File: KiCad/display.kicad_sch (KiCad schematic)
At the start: 30 parts, among them IC2 R1200N001A-TR-FE, J3 Conn_01x34_NHD_18, Q3 DMG2302U, Q4 DMG2302U, U6 MCP1700x-250xxTT

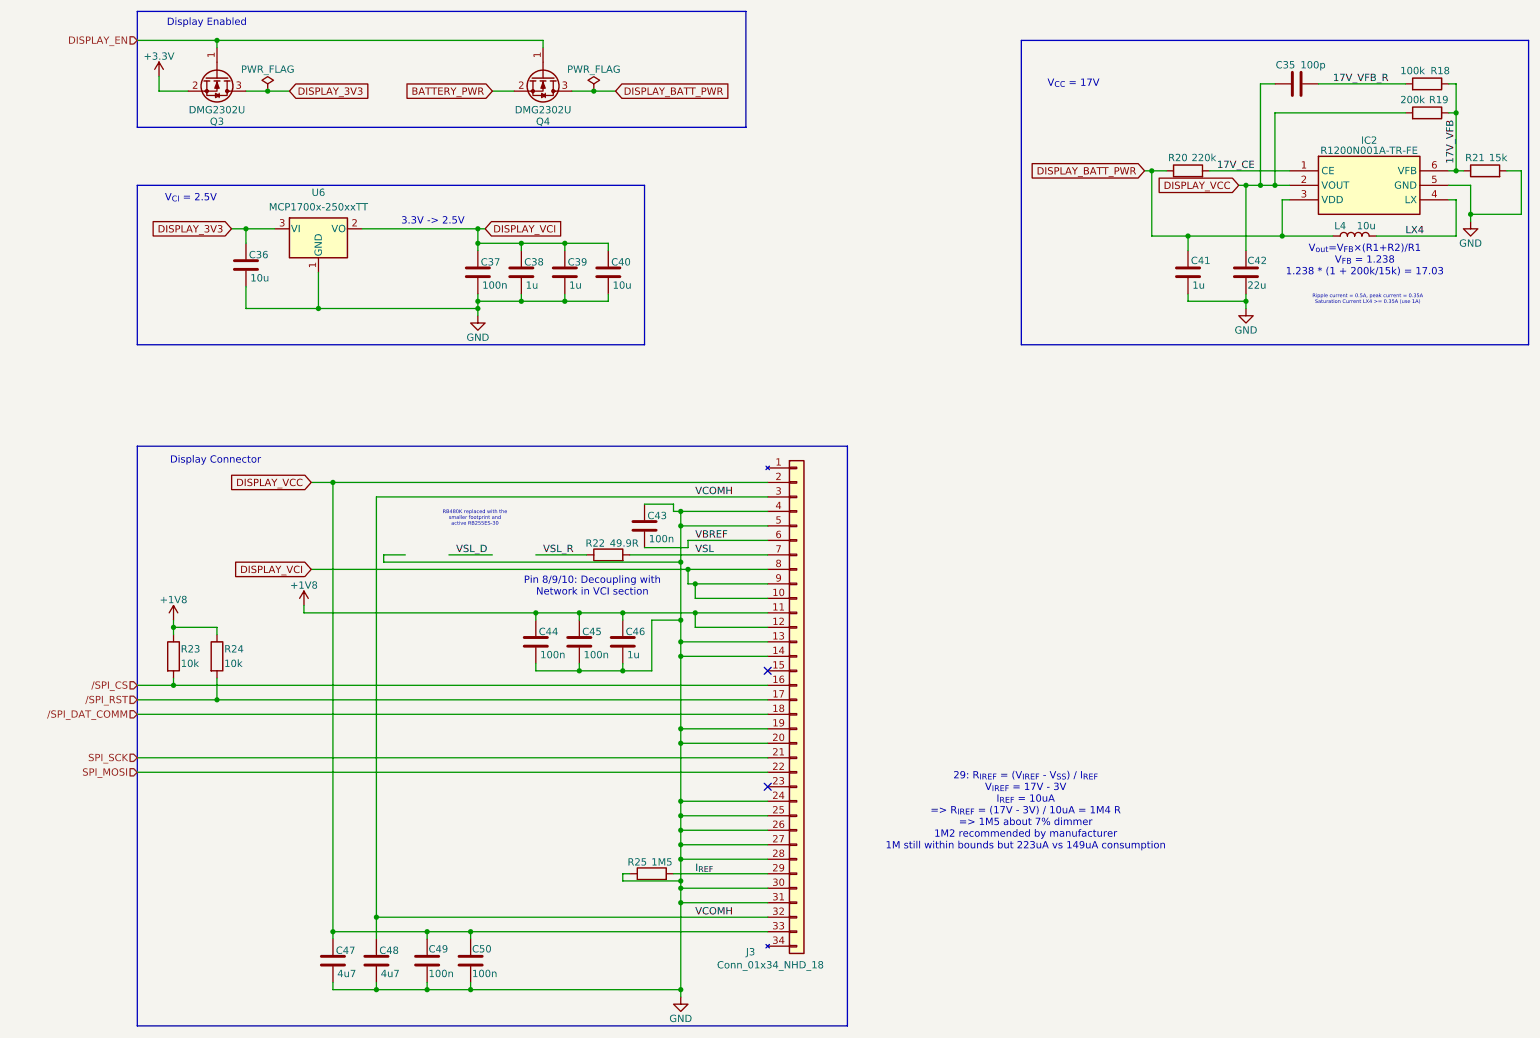
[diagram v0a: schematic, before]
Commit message: Implement Comments, Working on PCB Layout
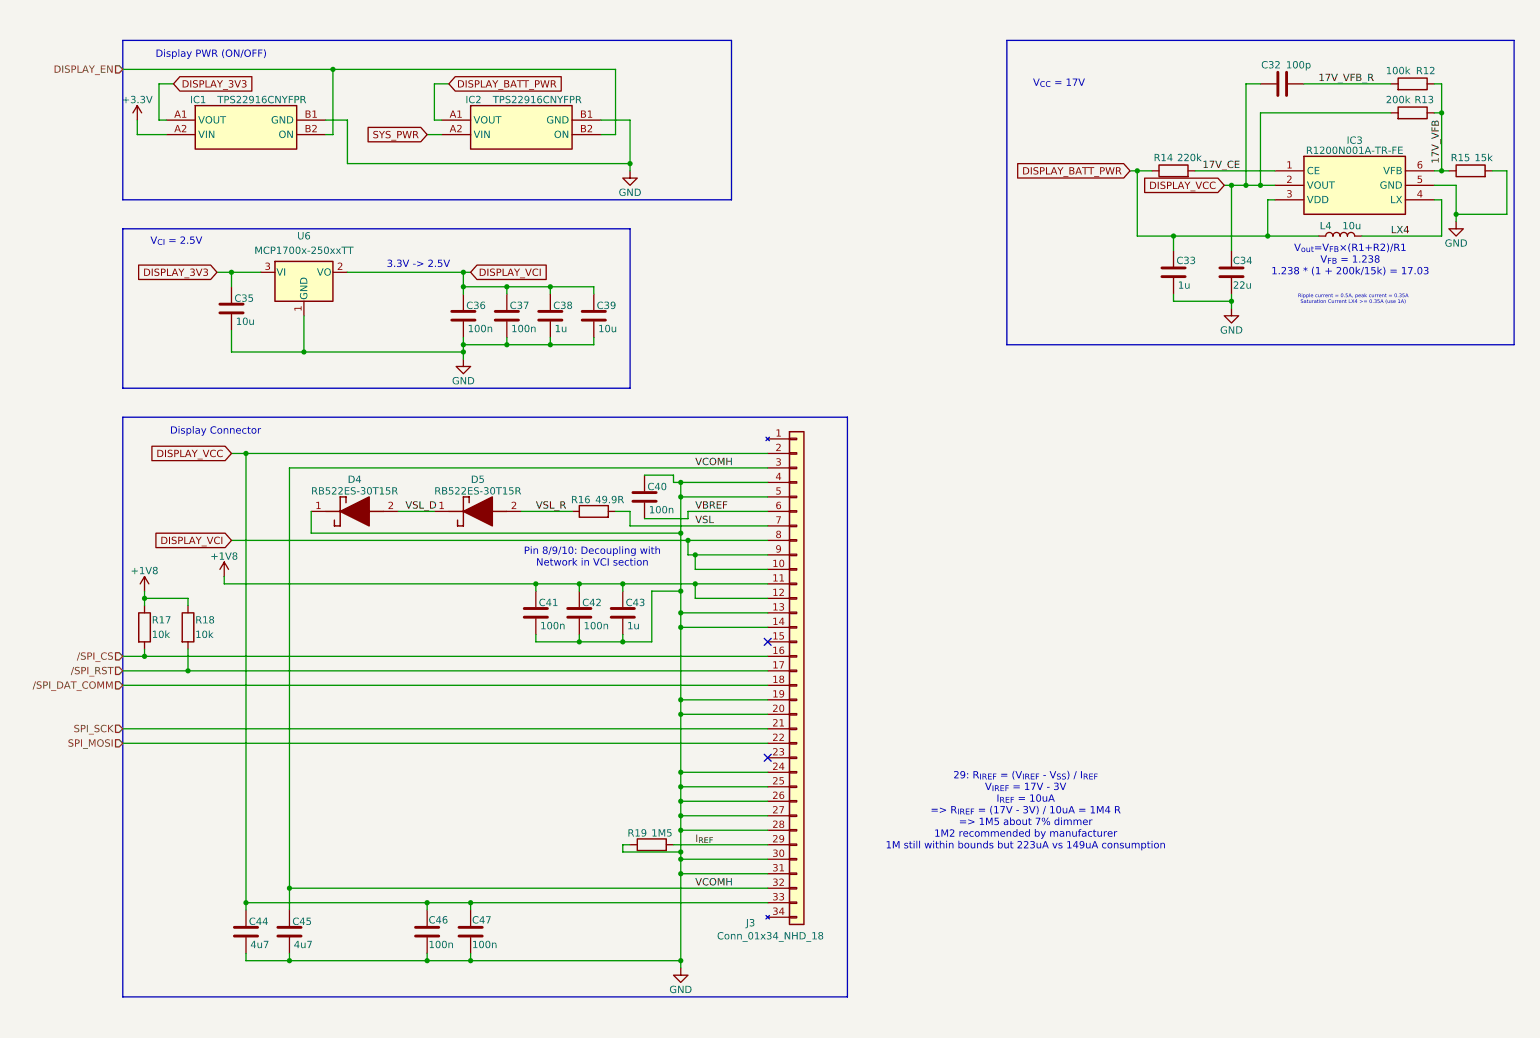
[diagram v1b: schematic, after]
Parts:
- removed Q3, Q4: DMG2302U, Package_TO_SOT_SMD:SOT-23, symbol Transistor_FET:DMG2302U
- added D4, D5: RB522ES-30T15R, RB522ES-30T15R:RB522ES30, symbol RB522ES-30T15R:RB522ES-30T15R
- added IC1, IC2: TPS22916CNYFPR, TPS22916CNYFPR:BGA4C40P2X2_78X78X50, symbol TPS22916CNYFPR:TPS22916CNYFPR
- C37: renamed from C38; value 1u -> 100n
- renumbered C35 to C32, C41 to C33, C42 to C34, C36 to C35, C37 to C36, C39 to C38, C40 to C39, C43 to C40, C44 to C41, C45 to C42, C46 to C43, C47 to C44, C48 to C45, C49 to C46, C50 to C47, IC2 to IC3, R18 to R12, R19 to R13, R20 to R14, R21 to R15, R22 to R16, R23 to R17, R24 to R18, R25 to R19
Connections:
- net +3.3V: now also IC1.A2 (VIN)
- net DISPLAY_3V3: now also IC1.A1 (VOUT)
- net DISPLAY_BATT_PWR: now also IC2.A1 (VOUT)
- net DISPLAY_EN: now also IC1.B2 (ON), IC2.B2 (ON)
- net GND: now also D4.1 (K), IC1.B1 (GND), IC2.B1 (GND)
- net VSL_D: now also D4.2 (A), D5.1 (K)
- net VSL_R: now also D5.2 (A)
- new net SYS_PWR: IC2.A2 (VIN)
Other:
- note added: "Display PWR (ON/OFF)"
- note removed: "Display Enabled"
- note removed: "RB480K replaced with the smaller footprint and active RB255ES-30"
- moved on the sheet: C32, C33, C34, C35, C36, C37, C38, C39, C40, C41, C42, C43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
